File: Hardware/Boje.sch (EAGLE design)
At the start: 11 parts, among them IC1 AT-TINY85V, J1 POWER, J2 Free, J3 SWITCH

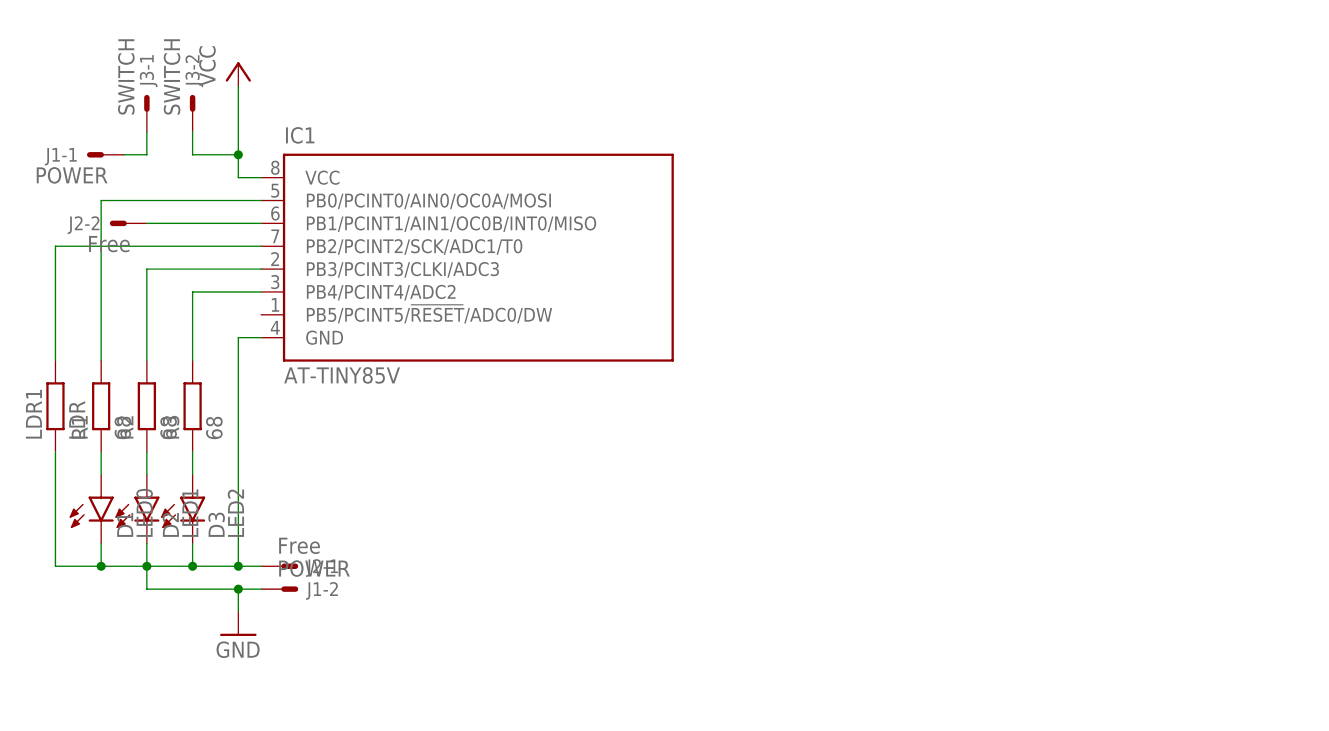
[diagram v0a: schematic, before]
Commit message: New PCB Layout
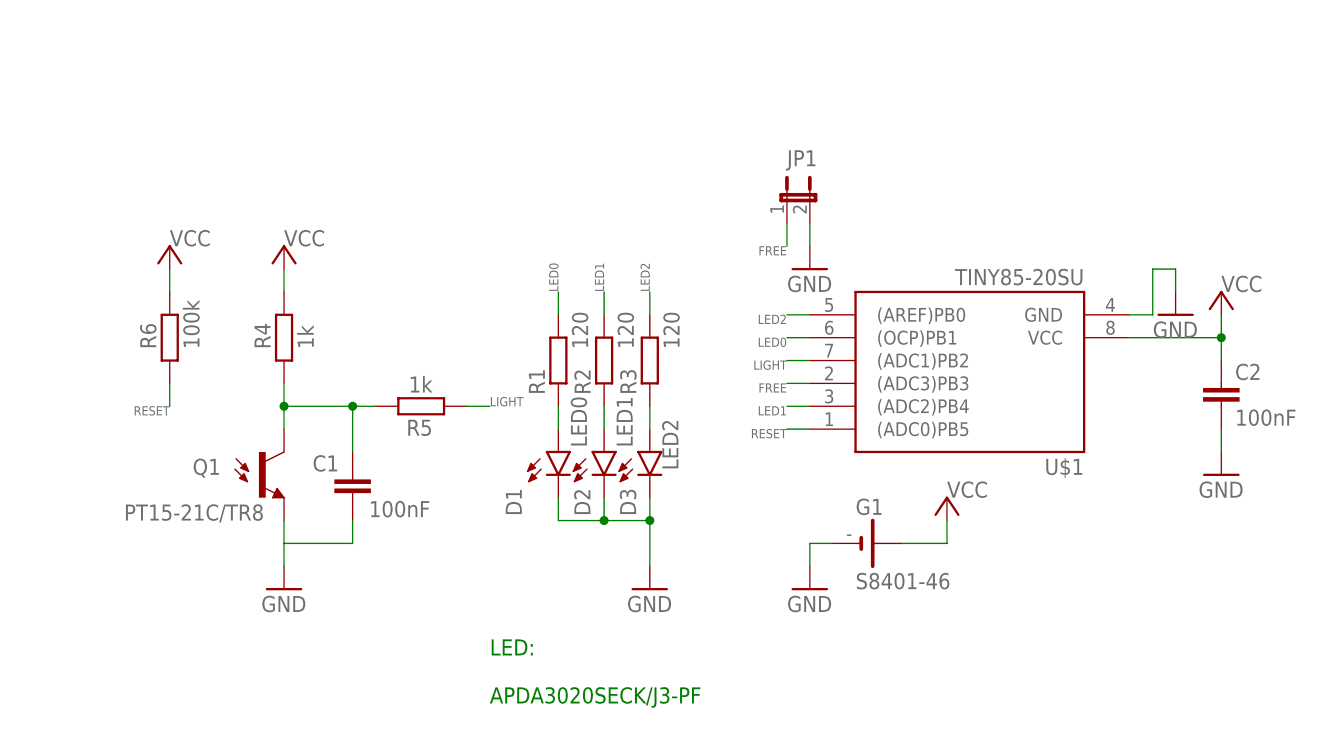
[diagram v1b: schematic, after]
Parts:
- removed IC1: AT-TINY85V, atmel:TINY13V-10PU
- removed J1: POWER, con-garry:332-02
- removed J2: Free, con-garry:332-02
- removed J3: SWITCH, con-garry:332-02
- removed LDR1: LDR, rcl:R-EU_V526-0
- added C1, C2: 100nF, rcl:C-EUC0603
- added G1: S8401-46, battery_holder:CR2032V
- added JP1: (no value), jumper:JP1E
- added Q1: PT15-21C/TR8, SparkFun-DiscreteSemi:PHOTOTRANSISTORPT17-21C-L41-TR8
- added R4, R5: 1k, rcl:R-EU_R0603
- added R6: 100k, rcl:R-EU_R0603
- added U$1: TINY85-20SU, avr-6:TINY25/45/85-20SU
- R1, R2, R3: value 68 -> 120; device resistor:R-EU_M2012 -> rcl:R-EU_R0603
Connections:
- removed net N$11: IC1.PB4/PCINT4/ADC2, R3.2
- removed net N$12: IC1.PB3/PCINT3/CLKI/ADC3, R2.2
- removed net N$13: IC1.PB0/PCINT0/AIN0/OC0A/MOSI, R1.2
- removed net N$14: IC1.PB2/PCINT2/SCK/ADC1/T0, LDR1.2
- removed net N$7: IC1.PB1/PCINT1/AIN1/OC0B/INT0/MISO, J2-2.S
- new net FREE: JP1.1, U$1.(ADC3)PB3
- new net LED0: R1.2, U$1.(OCP)PB1
- new net LED1: R2.2, U$1.(ADC2)PB4
- new net LED2: R3.2, U$1.(AREF)PB0
- new net LIGHT: R5.1, U$1.(ADC1)PB2
- new net RESET: R6.1, U$1.(ADC0)PB5
- net GND: now also C1.1, C2.2, G1.-, JP1.2, Q1.E, U$1.GND; no longer IC1.GND, J1-2.S, J2-1.S, LDR1.1
- net N$1: now also C1.2, Q1.C, R4.1, R5.2; no longer J1-1.S, J3-1.S
- net VCC: now also C2.1, G1.+, R4.2, R6.2, U$1.VCC; no longer IC1.VCC, J3-2.S
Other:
- note added: "LED: APDA3020SECK/J3-PF"
- moved on the sheet: D1, D2, D3, R1, R2, R3
